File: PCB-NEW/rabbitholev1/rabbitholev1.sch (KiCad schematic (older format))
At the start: 149 parts, among them SW1 SW_Push, U1 ATmega32U4-AU, Y1 Crystal_GND24_Small

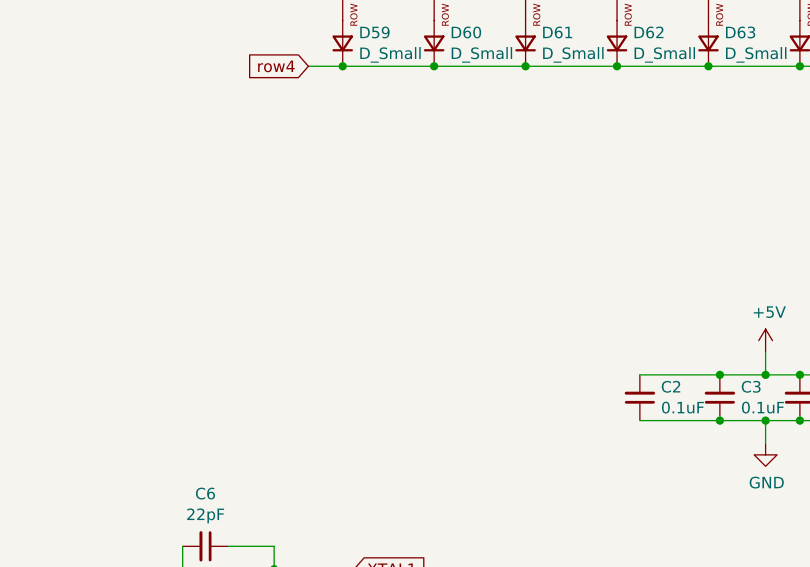
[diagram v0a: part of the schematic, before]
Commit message: d
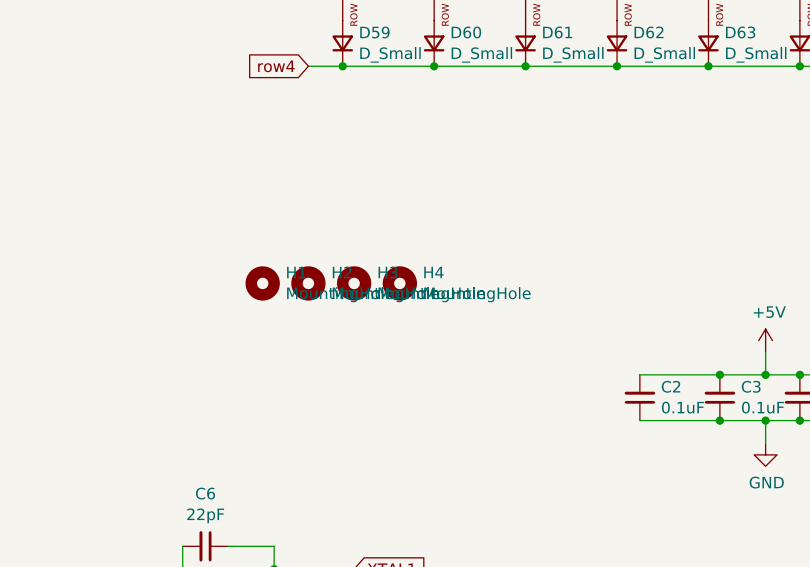
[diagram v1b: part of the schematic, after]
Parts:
- added H1, H2, H3, H4: MountingHole, symbol Mechanical:MountingHole
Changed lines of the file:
@@
 	11050 2300 11050 1650
 Connection ~ 11050 1650
+$Comp
+L Mechanical:MountingHole H1
+U 1 1 605F835A
+P 4900 4950
+F 0 "H1" H 5000 4996 50  0000 L CNN
+F 1 "MountingHole" H 5000 4905 50  0000 L CNN
+F 2 "" H 4900 4950 50  0001 C CNN
+F 3 "~" H 4900 4950 50  0001 C CNN
+	1    4900 4950
+	1    0    0    -1
+$EndComp
+$Comp
+L Mechanical:MountingHole H2
+U 1 1 605F8F1E
+P 5100 4950
+F 0 "H2" H 5200 4996 50  0000 L CNN
+F 1 "MountingHole" H 5200 4905 50  0000 L CNN
+F 2 "" H 5100 4950 50  0001 C CNN
+F 3 "~" H 5100 4950 50  0001 C CNN
+	1    5100 4950
+	1    0    0    -1
+$EndComp
+$Comp
+L Mechanical:MountingHole H3
+U 1 1 605F91A7
+P 5300 4950
+F 0 "H3" H 5400 4996 50  0000 L CNN
+F 1 "MountingHole" H 5400 4905 50  0000 L CNN
+F 2 "" H 5300 4950 50  0001 C CNN
+F 3 "~" H 5300 4950 50  0001 C CNN
+	1    5300 4950
+	1    0    0    -1
+$EndComp
+$Comp
+L Mechanical:MountingHole H4
+U 1 1 605F9444
+P 5500 4950
+F 0 "H4" H 5600 4996 50  0000 L CNN
+F 1 "MountingHole" H 5600 4905 50  0000 L CNN
+F 2 "" H 5500 4950 50  0001 C CNN
+F 3 "~" H 5500 4950 50  0001 C CNN
+	1    5500 4950
+	1    0    0    -1
+$EndComp
 $EndSCHEMATC

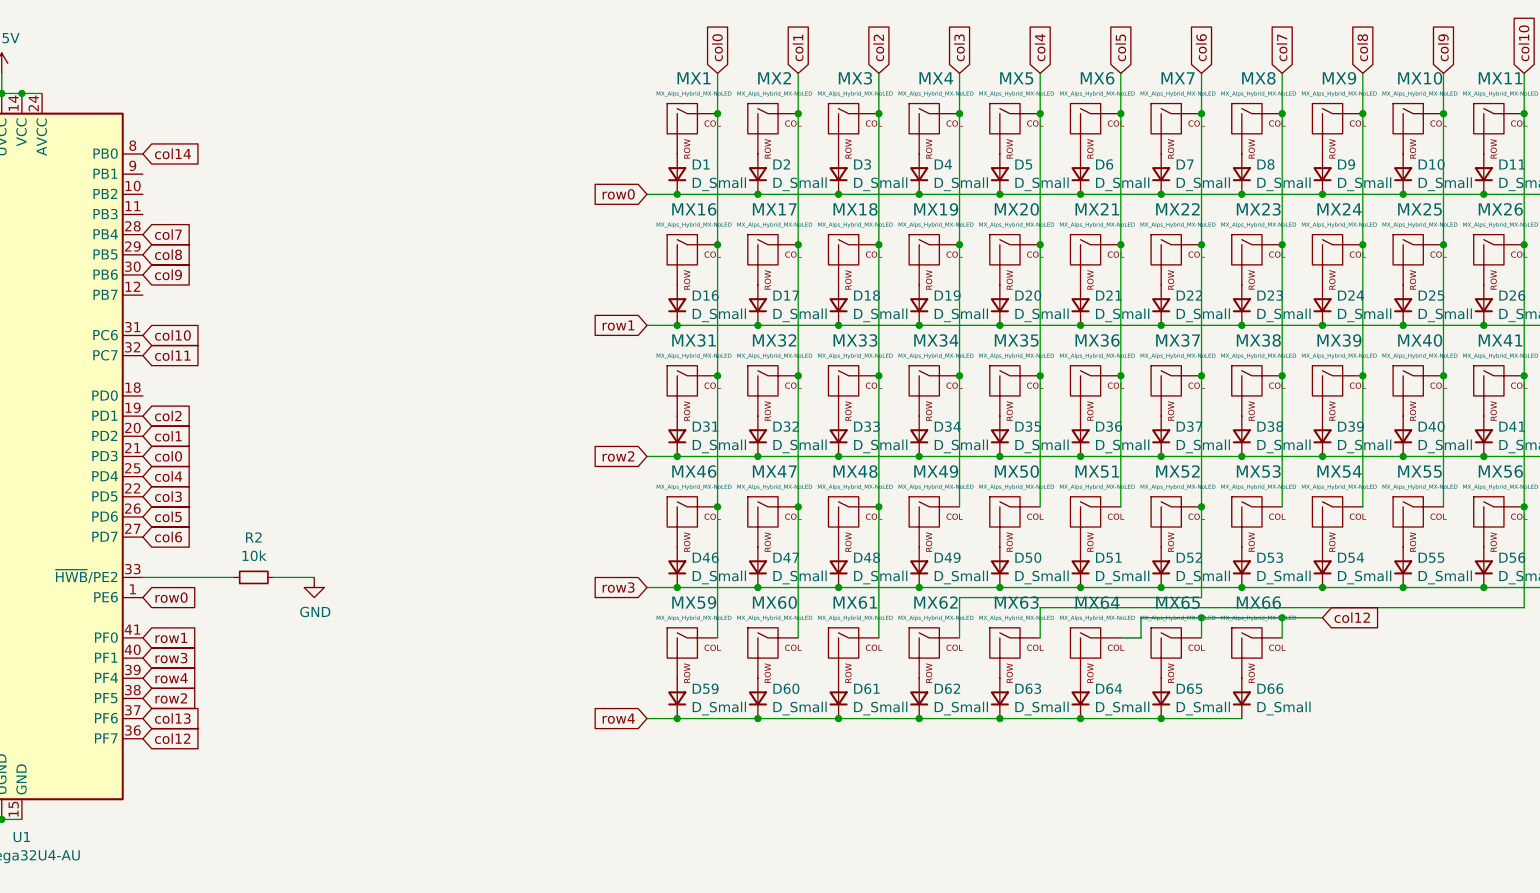
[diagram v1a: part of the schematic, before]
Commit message: f
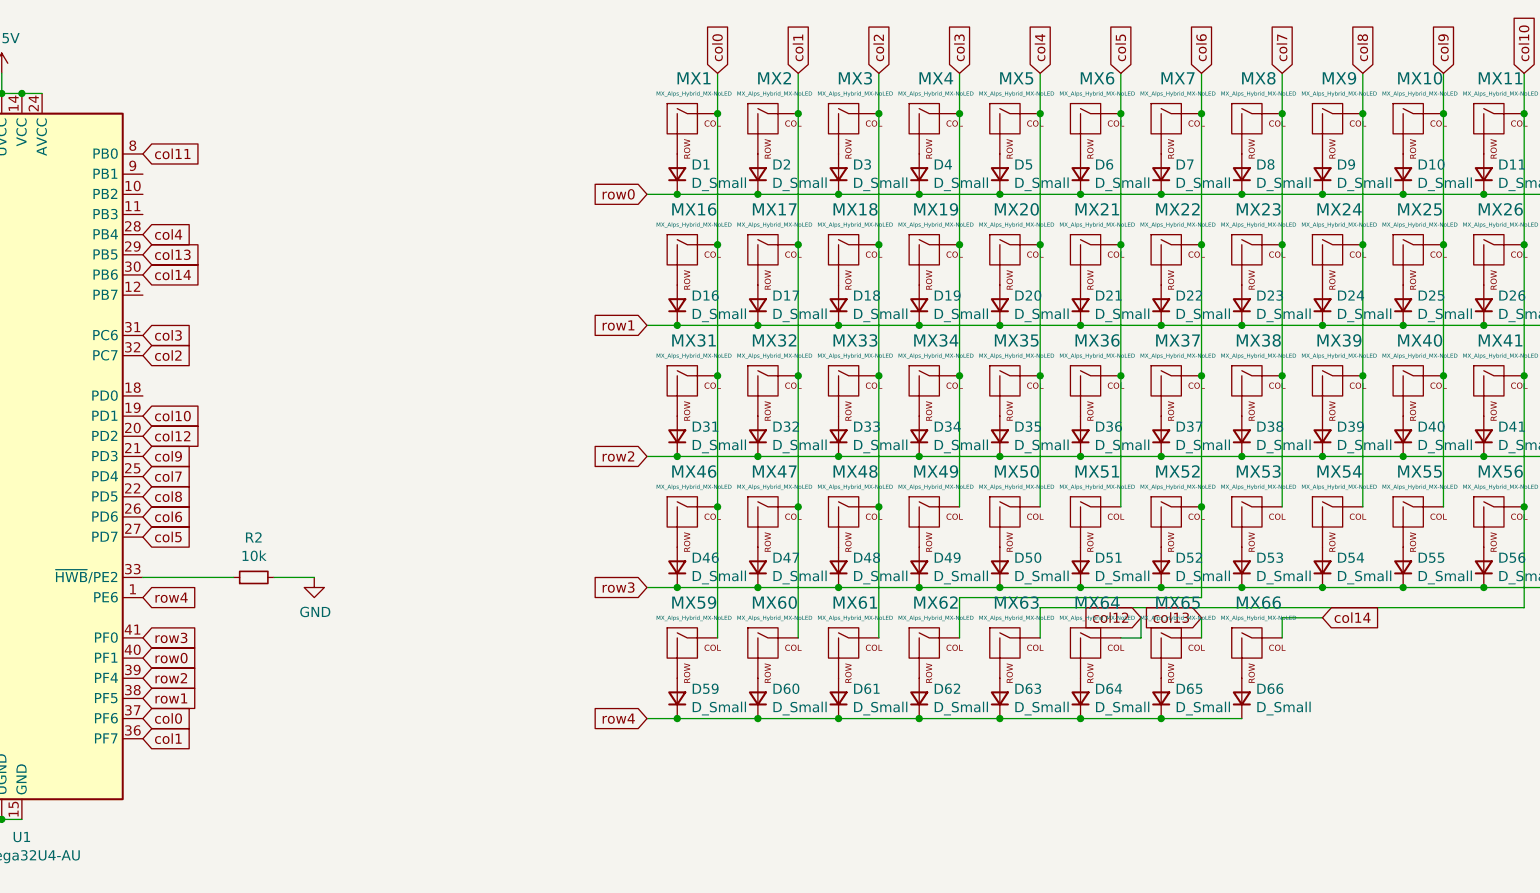
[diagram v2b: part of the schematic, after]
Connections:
- net col0: now also U1.37 (PF6); no longer U1.21 (PD3)
- net col1: now also U1.36 (PF7); no longer U1.20 (PD2)
- net col10: now also U1.19 (PD1); no longer U1.31 (PC6)
- net col11: now also U1.8 (PB0); no longer U1.32 (PC7)
- net col12: now also U1.20 (PD2); no longer MX65.1 (COL), MX66.1 (COL), U1.36 (PF7)
- net col13: now also MX65.1 (COL), U1.29 (PB5); no longer U1.37 (PF6)
- net col14: now also MX66.1 (COL), U1.30 (PB6); no longer U1.8 (PB0)
- net col2: now also U1.32 (PC7); no longer U1.19 (PD1)
- net col3: now also U1.31 (PC6); no longer U1.22 (PD5)
- net col4: now also U1.28 (PB4); no longer U1.25 (PD4)
- net col5: now also U1.27 (PD7); no longer U1.26 (PD6)
- net col6: now also U1.26 (PD6); no longer U1.27 (PD7)
- net col7: now also U1.25 (PD4); no longer U1.28 (PB4)
- net col8: now also U1.22 (PD5); no longer U1.29 (PB5)
- net col9: now also U1.21 (PD3); no longer U1.30 (PB6)
- net row0: now also U1.40 (PF1); no longer U1.1 (PE6)
- net row1: now also U1.38 (PF5); no longer U1.41 (PF0)
- net row2: now also U1.39 (PF4); no longer U1.38 (PF5)
- net row3: now also U1.41 (PF0); no longer U1.40 (PF1)
- net row4: now also U1.1 (PE6); no longer U1.39 (PF4)
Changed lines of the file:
@@
 	1    0    0    -1
 $EndComp
+Text GLabel 2600 4000 2    50   Input ~ 0
+col0
+Text GLabel 2600 4100 2    50   Input ~ 0
+col1
+Text GLabel 2600 2200 2    50   Input ~ 0
+col2
+Text GLabel 2600 2100 2    50   Input ~ 0
+col3
+Text GLabel 2600 1600 2    50   Input ~ 0
+col4
+Text GLabel 2600 2900 2    50   Input ~ 0
+col8
 Text GLabel 2600 2700 2    50   Input ~ 0
-col0
+col9
+Text GLabel 2600 2500 2    50   Input ~ 0
+col10
+Text GLabel 2600 1200 2    50   Input ~ 0
+col11
 Text GLabel 2600 2600 2    50   Input ~ 0
-col1
-Text GLabel 2600 2500 2    50   Input ~ 0
-col2
-Text GLabel 2600 2900 2    50   Input ~ 0
-col3
+col12
+Text GLabel 2600 1700 2    50   Input ~ 0
+col13
+Text GLabel 2600 1800 2    50   Input ~ 0
+col14
+Text GLabel 2600 3100 2    50   Input ~ 0
+col5
+Text GLabel 2600 3000 2    50   Input ~ 0
+col6
+Text GLabel 2600 3700 2    50   Input ~ 0
+row0
+Text GLabel 2600 3900 2    50   Input ~ 0
+row1
+Text GLabel 2600 3800 2    50   Input ~ 0
+row2
+Text GLabel 2600 3600 2    50   Input ~ 0
+row3
+Text GLabel 2600 3400 2    50   Input ~ 0
+row4
 Text GLabel 2600 2800 2    50   Input ~ 0
-col4
-Text GLabel 2600 1700 2    50   Input ~ 0
-col8
-Text GLabel 2600 1800 2    50   Input ~ 0
-col9
-Text GLabel 2600 2100 2    50   Input ~ 0
-col10
-Text GLabel 2600 2200 2    50   Input ~ 0
-col11
-Text GLabel 2600 4100 2    50   Input ~ 0
-col12
-Text GLabel 2600 4000 2    50   Input ~ 0
-col13
-Text GLabel 2600 1200 2    50   Input ~ 0
-col14
-Text GLabel 2600 3000 2    50   Input ~ 0
-col5
-Text GLabel 2600 3100 2    50   Input ~ 0
-col6
-Text GLabel 2600 3400 2    50   Input ~ 0
-row0
-Text GLabel 2600 3600 2    50   Input ~ 0
-row1
-Text GLabel 2600 3900 2    50   Input ~ 0
-row2
-Text GLabel 2600 3700 2    50   Input ~ 0
-row3
-Text GLabel 2600 3800 2    50   Input ~ 0
-row4
-Text GLabel 2600 1600 2    50   Input ~ 0
 col7
 Wire Wire Line
@@
 	7550 3600 7550 3500
 Wire Wire Line
-	7550 3500 7850 3500
-Wire Wire Line
 	7850 3600 7850 3500
-Connection ~ 7850 3500
-Wire Wire Line
-	7850 3500 8250 3500
 Wire Wire Line
 	8250 3600 8250 3500
-Connection ~ 8250 3500
 Wire Wire Line
 	10250 2300 10250 1650
 Wire Wire Line
 	8250 3500 8450 3500
-Text GLabel 8450 3500 2    50   Input ~ 0
-col12
 Wire Wire Line
 	10700 2950 10700 1650
@@
 	1    0    0    -1
 $EndComp
+Text GLabel 7550 3500 0    50   Input ~ 0
+col12
+Text GLabel 7850 3500 0    50   Input ~ 0
+col13
+Text GLabel 8450 3500 2    50   Input ~ 0
+col14
 $EndSCHEMATC
